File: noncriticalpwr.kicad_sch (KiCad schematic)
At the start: 2 parts, among them J4 Power Conn

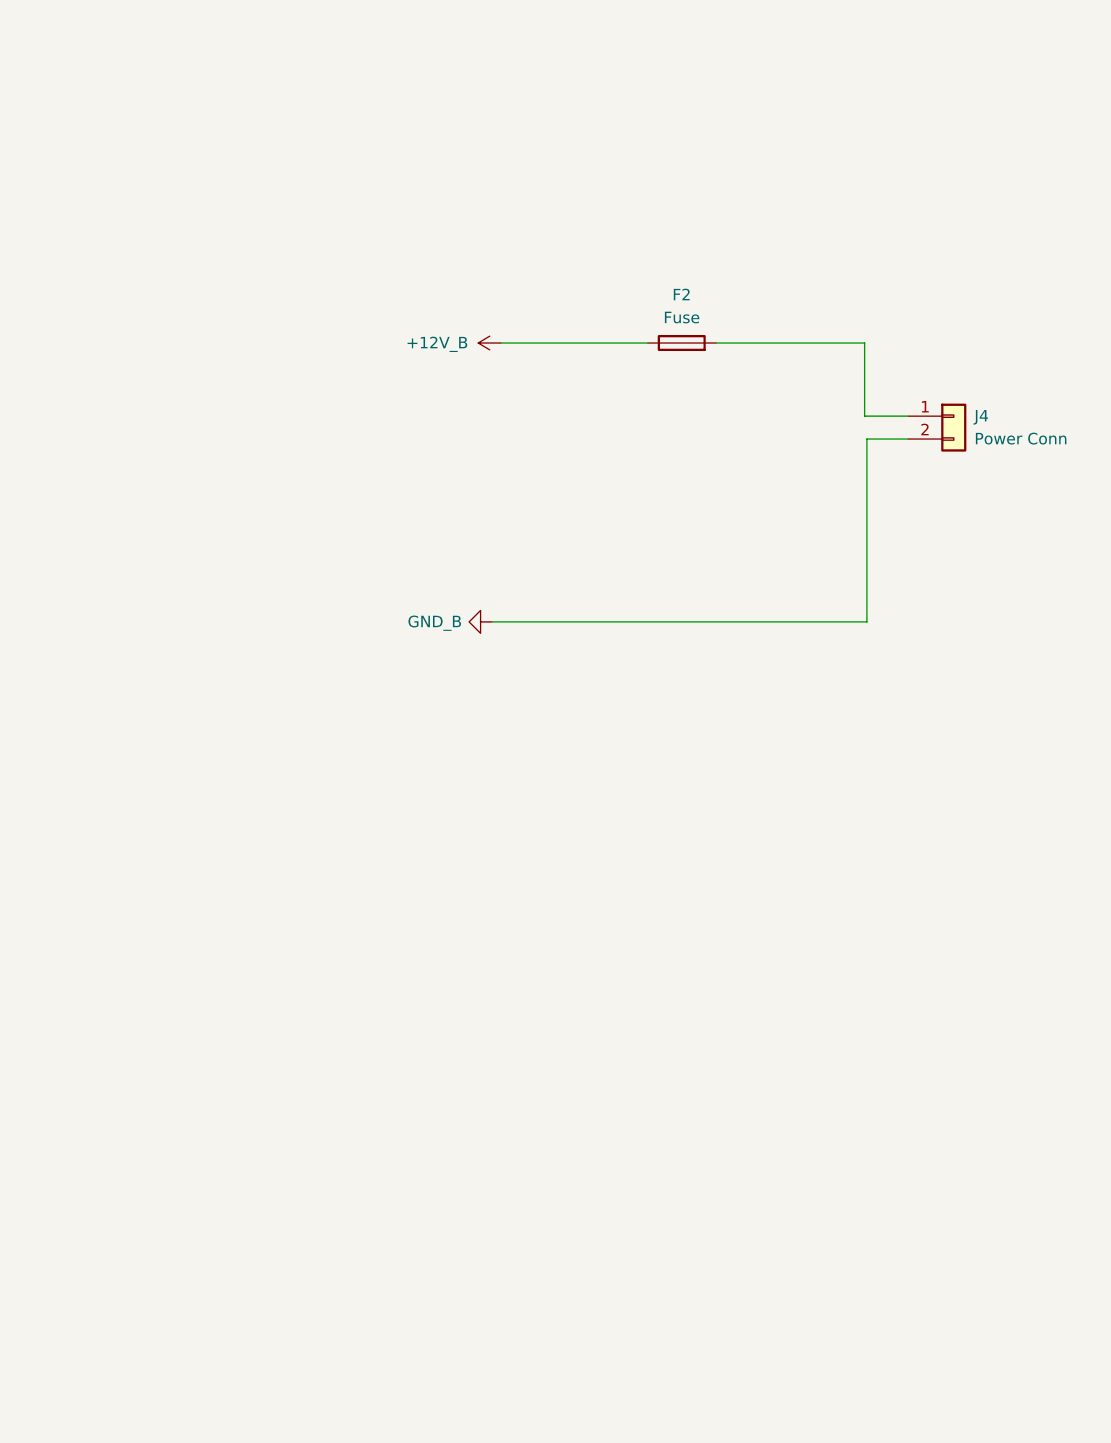
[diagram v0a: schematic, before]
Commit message: finished schematic
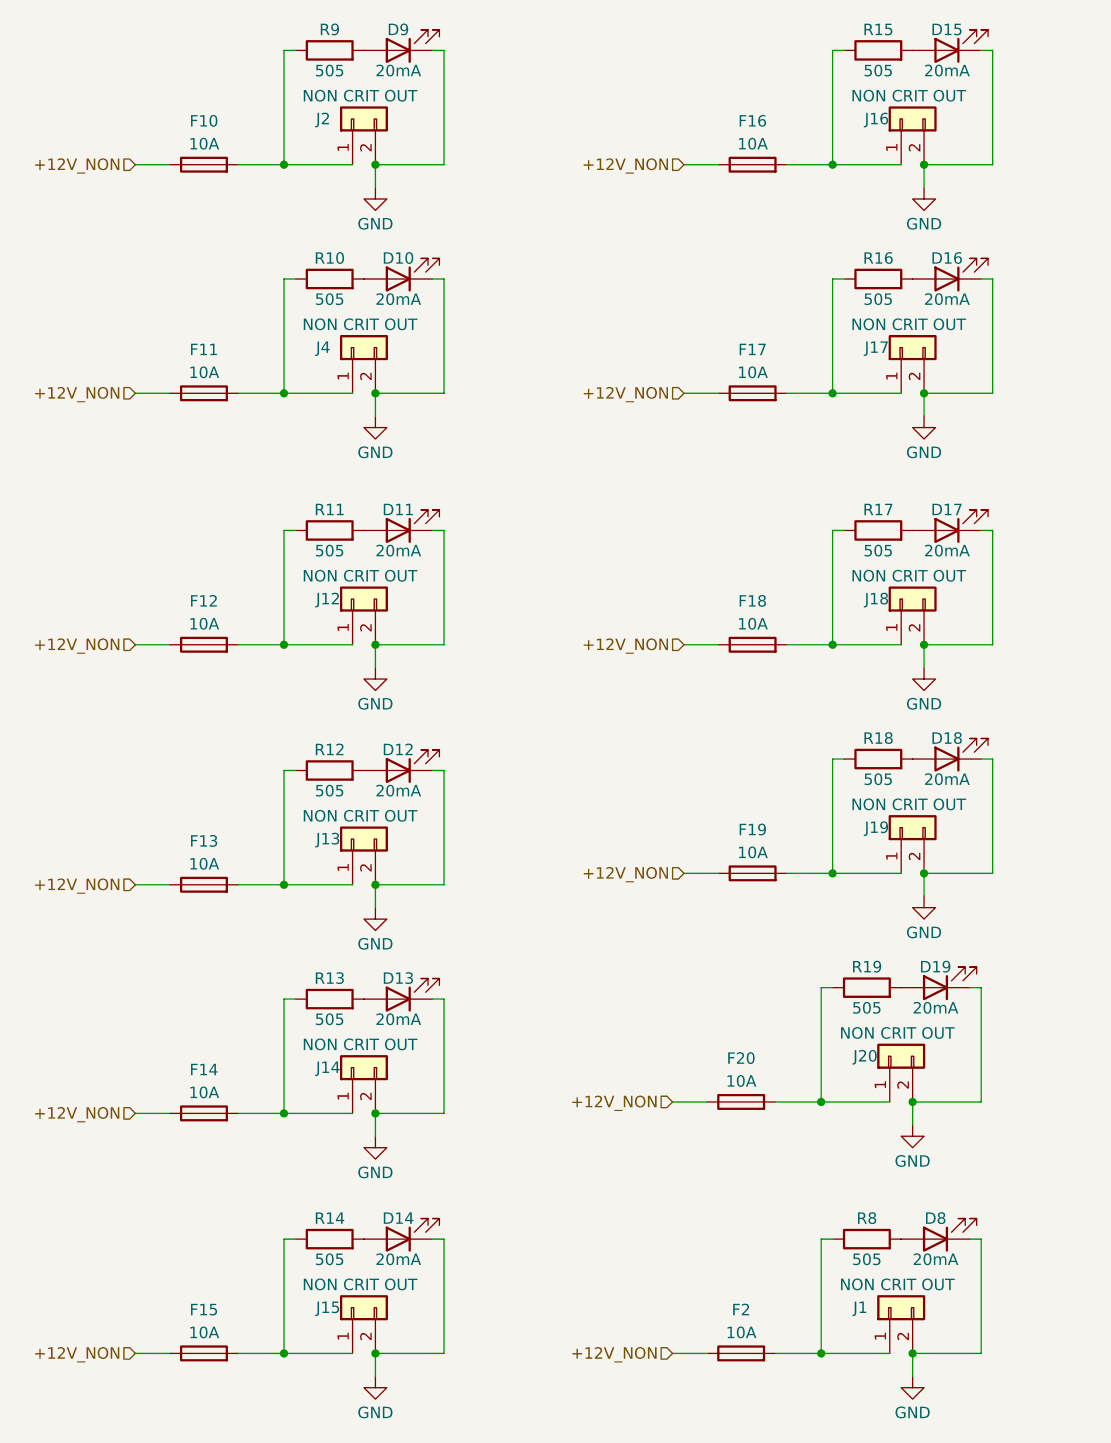
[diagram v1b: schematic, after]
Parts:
- added D10, D11, D12, D13, D14, D15, D16, D17, D18, D19, D8, D9: 20mA, LED_SMD:LED_0805_2012Metric, symbol Device:LED
- added F10, F11, F12, F13, F14, F15, F16, F17, F18, F19, F20: 10A, footprints:3588, symbol Device:Fuse
- added J1, J12, J13, J14, J15, J16, J17, J18, J19, J2, J20: NON CRIT OUT, footprints:Molex_Micro-Fit_3.0_43650-0215_1x02_P3.00mm_Vertical, symbol Connector_Generic:Conn_01x02
- added R10, R11, R12, R13, R14, R15, R16, R17, R18, R19, R8, R9: 505, Resistor_SMD:R_0805_2012Metric, symbol Device:R
- F2: value Fuse -> 10A
- J4: value Power Conn -> NON CRIT OUT
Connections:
- net at F2.2: now also J1.1 (Pin_1), R8.1; no longer J4.1 (Pin_1)
- net +12V_B renamed +12V_NON
- net +12V_NON: now also F10.1, F11.1, F12.1, F13.1, F14.1, F15.1, F16.1, F17.1, F18.1, F19.1, F20.1
- net GND_B renamed GND
- net GND: now also D10.1 (K), D11.1 (K), D12.1 (K), D13.1 (K), D14.1 (K), D15.1 (K), D16.1 (K), D17.1 (K), D18.1 (K), D19.1 (K), D8.1 (K), D9.1 (K), J1.2 (Pin_2), J12.2 (Pin_2), J13.2 (Pin_2), J14.2 (Pin_2), J15.2 (Pin_2), J16.2 (Pin_2), J17.2 (Pin_2), J18.2 (Pin_2), J19.2 (Pin_2), J2.2 (Pin_2), J20.2 (Pin_2)
- new net: F13.2, J13.1 (Pin_1), R12.1
- new net: D13.2 (A), R13.2
- new net: F14.2, J14.1 (Pin_1), R13.1
- new net: F20.2, J20.1 (Pin_1), R19.1
- new net: F12.2, J12.1 (Pin_1), R11.1
- new net: F10.2, J2.1 (Pin_1), R9.1
- new net: D19.2 (A), R19.2
- new net: D17.2 (A), R17.2
- new net: F19.2, J19.1 (Pin_1), R18.1
- new net: F15.2, J15.1 (Pin_1), R14.1
- new net: D15.2 (A), R15.2
- new net: D11.2 (A), R11.2
- new net: F16.2, J16.1 (Pin_1), R15.1
- new net: D8.2 (A), R8.2
- new net: F17.2, J17.1 (Pin_1), R16.1
- new net: D16.2 (A), R16.2
- new net: D14.2 (A), R14.2
- new net: D18.2 (A), R18.2
- new net: D12.2 (A), R12.2
- new net: F11.2, J4.1 (Pin_1), R10.1
- new net: D10.2 (A), R10.2
- new net: D9.2 (A), R9.2
- new net: F18.2, J18.1 (Pin_1), R17.1
